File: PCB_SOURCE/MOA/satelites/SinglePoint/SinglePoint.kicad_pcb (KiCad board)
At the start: 2 copper layers, 30 x 23 mm, 9 parts, among them J1 Conn_01x04, SW1 6mm_tactile

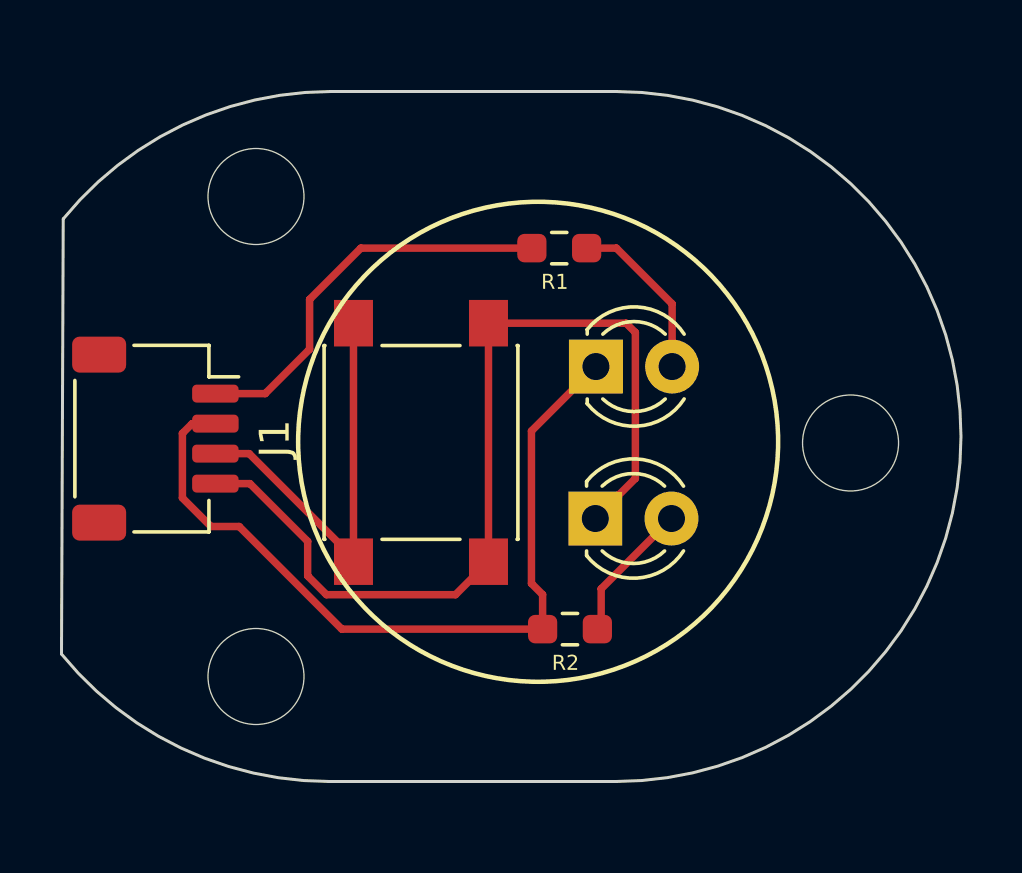
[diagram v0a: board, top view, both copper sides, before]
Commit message: added some files, but mainly this is to update hex file of OSSD
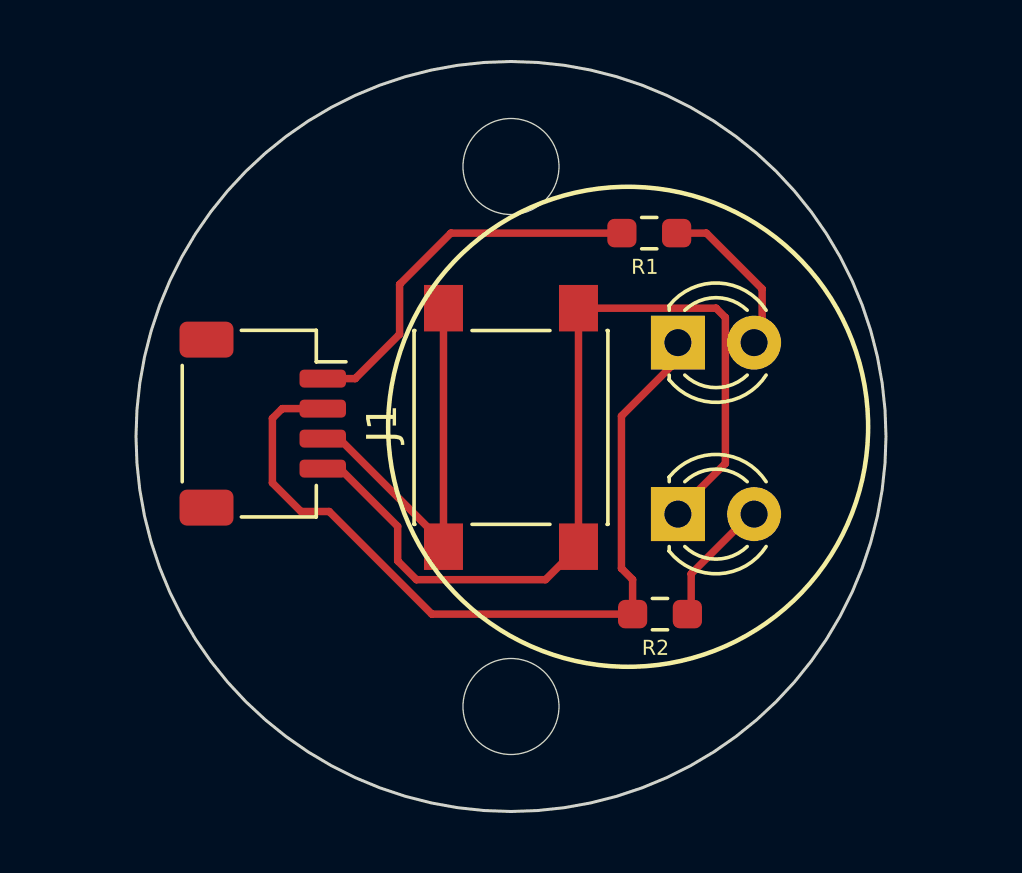
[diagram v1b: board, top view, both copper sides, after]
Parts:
- removed the REF** at (51.8, 61.2)
- moved REF** 8.56 mm to (40.5, 52.0)
- moved REF** 8.56 mm to (40.5, 70.0)
- moved J1 3.61 mm to (32.2, 60.6)
- moved R1 3.04 mm to (45.1, 54.2)
- moved R2 3.04 mm to (45.5, 66.9)
- moved SW1 3.04 mm to (40.5, 60.7)
- moved D1 2.85 mm to (46.1, 57.9)
- moved D2 2.76 mm to (46.1, 63.6)
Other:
- board size 30 x 23 mm -> 25 x 25 mm
